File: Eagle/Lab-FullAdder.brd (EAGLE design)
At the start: 50 x 50 mm, 69 parts, among them CN1 HD2, Q1 2N3904-1, Q10 2N3904-1, Q11 2N3904-1, Q12 2N3904-1, Q13 2N3904-1, Q14 2N3904-1, Q15 2N3904-1, Q16 2N3904-1, Q17 BC557BH, Q18 BC557BH, Q2 2N3904-1, Q3 2N3904-1, Q4 2N3904-1, Q5 2N3904-1, Q6 2N3904-1, Q7 2N3904-1, Q8 BC557BH, Q9 BC557BH

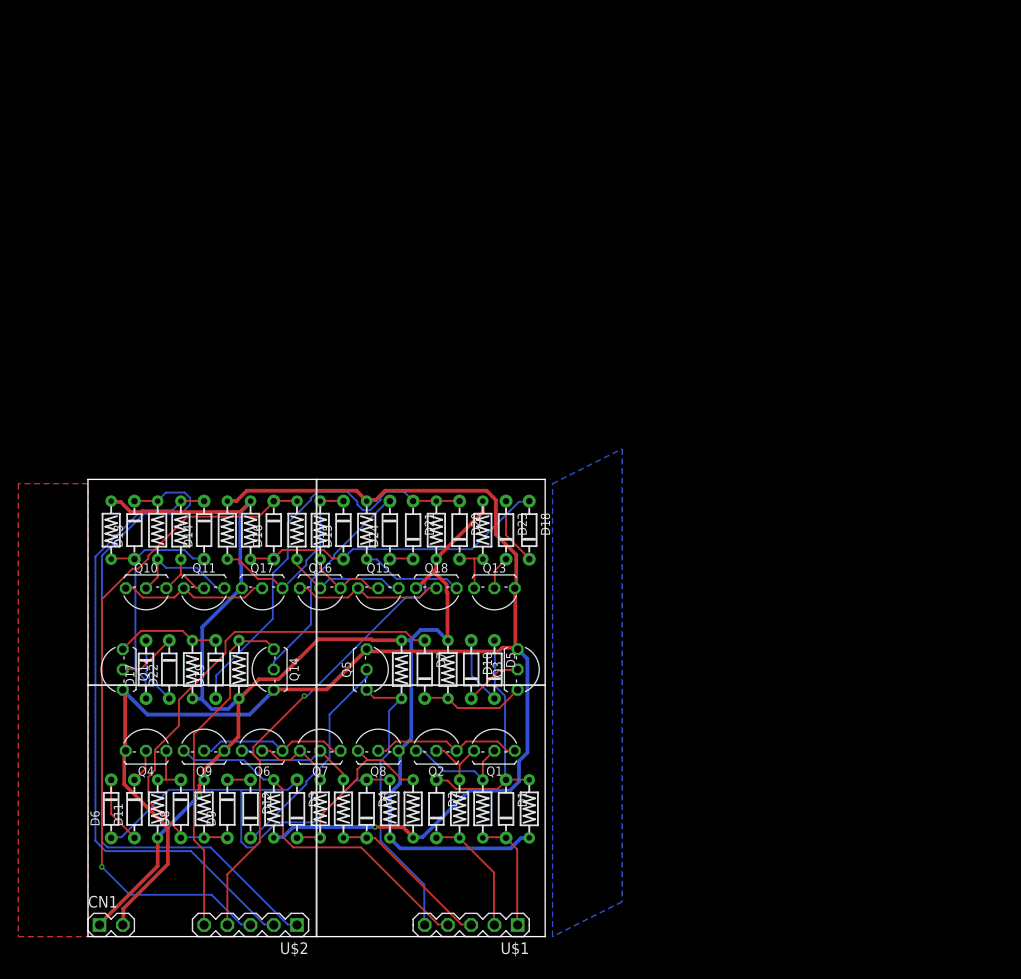
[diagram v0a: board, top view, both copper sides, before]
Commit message: General flush of files
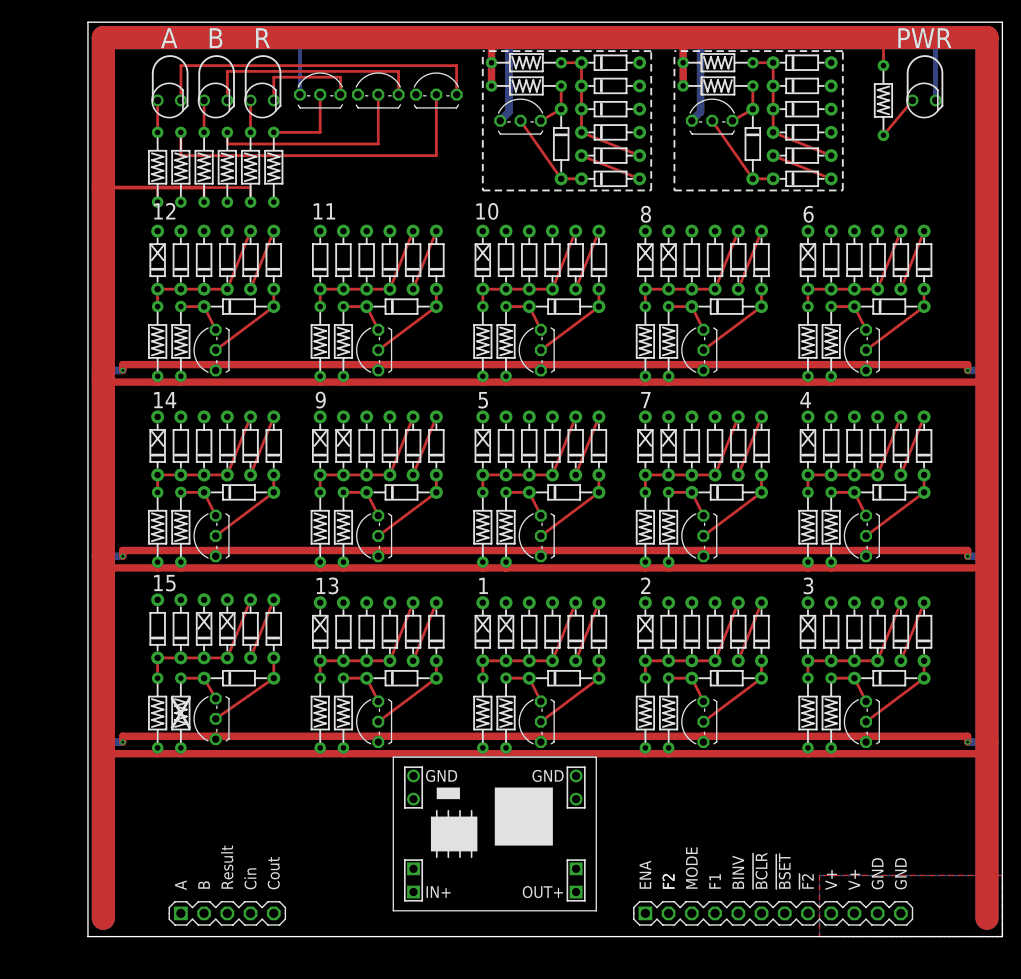
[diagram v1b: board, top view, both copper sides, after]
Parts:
- removed U$2: HD5CN, SmallRoomLabs_ConSwitch:HD5
- added D100, D101, D102, D104, D105, D106, D107, D108, D109, D110, D111, D112, D113, D114, D115, D116, D117, D118, D119, D25, D26, D27, D28, D30, D31, D32, D33, D34, D36, D37, D38, D39, D40, D43, D44, D45, D46, D47, D49, D50, D51, D52, D53, D55, D56, D57, D58, D59, D62, D63, D64, D65, D66, D68, D69, D70, D71, D72, D74, D75, D76, D77, D78, D80, D81, D82, D83, D84, D85, D86, D87, D88, D89, D90, D92, D93, D94, D95, D96, D98, D99: DIODE-6.3, SmallRoomLabs_Semiconductor:DO35-6.3
- added D103, D29, D35, D41, D42, D48, D54, D60, D61, D67, D73, D79, D91, D97: DIODE-7.6, SmallRoomLabs_Semiconductor:DO35-7.6
- added LD1, LD2, LD3, LD4: LED-RA, SmallRoomLabs_Led:3MMRA
- added Q19, Q20: 2N3904-1, SmallRoomLabs_Semiconductor:TO92BH
- added R25, R26, R27, R28, R29, R30, R31, R32, R33, R34, R35, R38, R39, R40, R41, R42, R43: R1/8-7.6MM, SmallRoomLabs_Discrete:R0125-7.6
- added VR1: SMPS, SmallRoomLabs_Battery:BUCK1722
- CN1: value HD2 -> HD12; device SmallRoomLabs_ConSwitch:HD2 -> SmallRoomLabs_ConSwitch:HD12
- D11, D17, D23: value DIODE-6.3 -> DIODE-7.6; device SmallRoomLabs_Semiconductor:DO35-6.3 -> SmallRoomLabs_Semiconductor:DO35-7.6
- Q17, Q18, Q8, Q9: value BC557BH -> 2N3904-1
- R1, R10, R11, R12, R13, R14, R15, R16, R17, R18, R19, R2, R20, R21, R22, R23, R24, R3, R4, R5, R6, R7, R8, R9: value R1/8-6MM -> R1/8-7.6MM; device SmallRoomLabs_Discrete:R0125-6.3 -> SmallRoomLabs_Discrete:R0125-7.6
- moved D22 86.1 mm to (91.4, 53.7), turned to 270 degrees
- moved Q4 82.2 mm to (85.1, 43.8), turned to 90 degrees
- moved D17 81.3 mm to (87.6, 28.3), turned to 180 degrees
- moved D13 79.5 mm to (83.8, 33.3), turned to 270 degrees
- moved Q6 79.3 mm to (85.1, 64.1), turned to 90 degrees
- moved R10 77.5 mm to (78.7, 44.8)
- moved R11 75.2 mm to (81.3, 44.8), turned to 270 degrees
- moved D14 74.5 mm to (86.4, 33.3), turned to 270 degrees
- moved D19 74.0 mm to (83.8, 53.7), turned to 270 degrees
- moved CN1 72.4 mm to (74.9, 2.54)
- moved D16 72.0 mm to (91.4, 33.3), turned to 270 degrees
- moved R17 69.2 mm to (81.3, 65.1), turned to 270 degrees
- moved D12 66.4 mm to (81.3, 33.3)
- moved D11 66.3 mm to (69.8, 28.3), turned to 180 degrees
- moved R16 64.4 mm to (78.7, 65.1)
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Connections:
- removed net A2: D13.C, R14.2, U$2.P$1
- removed net B2: D14.C, R15.2, U$2.P$2
- removed net CI: D4.C, R7.1, U$1.P$3
- removed net CI2: D16.C, R19.1, U$2.P$3
- removed net CO: Q5.3, R12.1, U$1.P$5
- removed net CO2: Q14.3, R24.1, U$2.P$5
- removed net N$19: D11.C, Q4.2
- removed net S: Q9.1, R8.2, U$1.P$4
- removed net S2: Q18.1, R20.2, U$2.P$4
- new net !BCLR: CN1.P$6, D14.A, D7.A
- new net !BSET: CN1.P$7, D20.A
- new net !F2: CN1.P$8, D32.A
- new net BINV: CN1.P$5, D12.A, D2.A
- new net CIN: D36.A, D55.A, U$1.P$4
- new net COUT: D73.C, Q13.3, R18.1, U$1.P$5
- new net ENA: CN1.P$1, D68.A, D98.A
- new net F1: CN1.P$4, D25.A
- new net F2: CN1.P$2, D113.A, D63.A
- new net G10OUT: D114.A, D60.C, D62.A, D69.A, Q10.3, R29.1
- new net G11OUT: D61.C, D74.A, Q11.3, R6.1
- new net G12OUT: D67.C, D75.A, Q12.3, R12.1
- new net G14OUT: D119.A, D79.C, Q14.3, R24.1
- new net G1OUT: D13.A, D41.C, D8.A, Q1.3, R3.1
- new net G2OUT: D11.C, D18.A, Q2.3, R5.1
- new net G3OUT: D17.C, D19.A, Q3.3, R8.1
- new net G4OUT: D23.C, D26.A, D31.A, D45.A, Q4.3, R11.1
- new net G5OUT: D29.C, D38.A, D44.A, D70.A, Q5.3, R14.1
- new net G6OUT: D35.C, D76.A, Q6.3, R17.1
- new net G7OUT: D42.C, D50.A, Q7.3, R20.1
- new net G8OUT: D48.C, D51.A, Q8.3, R23.1
- new net G9OUT: D54.C, D57.A, D64.A, Q9.3, R26.1
- new net MODE: CN1.P$3, D3.A, D56.A
- new net N$37: D27.C, D28.A
- new net N$38: D28.C, D29.A, Q5.2
- new net N$39: D87.A
- new net N$40: D88.A
- new net N$41: D81.A
- new net N$42: D117.C, D86.C, D87.C, D88.C, D89.A, R38.1
- new net N$43: D89.C, D90.A
- new net N$44: D109.C, D30.C, D31.C, D32.C, D33.A, R16.1
- new net N$45: D33.C, D34.A
- new net N$46: D34.C, D35.A, Q6.2
- new net N$47: D90.C, D91.A, Q19.2
- new net N$48: D118.C, D92.C, D93.C, D94.C, D95.A, R40.1
- new net N$49: D95.C, D96.A
- new net N$50: D96.C, D97.A, Q20.2
- new net N$51: D100.C, D101.A, D119.C, D98.C, D99.C, R42.1
- new net N$52: D112.C, D37.C, D38.C, D39.A, D83.C, R19.1
- new net N$53: D39.C, D40.A
- new net N$54: D40.C, D42.A, Q7.2
- new net N$55: D101.C, D102.A
- new net N$56: D102.C, D103.A, Q15.2
- new net N$57: D115.C, D62.C, D63.C, D64.C, D65.A, R9.1
- new net N$58: D82.A
- new net N$59: D83.A
- new net N$60: D110.C, D44.C, D45.C, D46.A, D81.C, R22.1
- new net N$61: D46.C, D47.A
- new net N$62: D47.C, D48.A, Q8.2
- new net N$63: D85.A
- new net N$64: D65.C, D66.A
- new net N$65: D66.C, D67.A, Q12.2
- new net N$66: D84.A
- new net N$67: D104.A
- new net N$68: D111.C, D50.C, D51.C, D52.A, D82.C, R25.1
- new net N$69: D52.C, D53.A
- new net N$70: D53.C, D54.A, Q9.2
- new net N$71: D105.A
- new net N$72: D106.A
- new net N$73: D108.A
- new net N$74: D107.A
- new net N$75: D109.A
- new net N$76: D104.C, D55.C, D56.C, D57.C, D58.A, R28.1
- new net N$77: D58.C, D59.A
- new net N$78: D59.C, D60.A, Q10.2
- new net N$79: D110.A
- new net N$80: D111.A
- new net N$81: D112.A
- new net N$82: D116.C, D68.C, D69.C, D70.C, D71.A, R15.1
- new net N$83: D71.C, D72.A
- new net N$84: D72.C, D73.A, Q13.2
- new net N$85: D116.A
- new net N$86: D115.A
- new net N$88: D118.A
- new net N$89: D74.C, D75.C, D76.C, D77.A, D80.C, R21.1
- new net N$90: D77.C, D78.A
- new net N$91: D78.C, D79.A, Q14.2
- new net N$92: D117.A
- new net RES: D103.C, Q15.3, R33.2, R43.1, U$1.P$3
- new net VIN: VR1.IN@1, VR1.IN@2
- new net VOUT: VR1.OUT@1, VR1.OUT@2
- net A: now also D24.A, D30.A, D37.A, R35.2; no longer D1.C, R2.2
- net B: now also D1.A, D6.A, R34.2; no longer D2.C, R3.2
- net GND: now also CN1.P$11, CN1.P$12, LD4.C, Q1.1, Q10.1, Q11.1, Q15.1, Q16.1, Q17.1, Q18.1, Q19.1, Q2.1, Q20.1, Q6.1, Q7.1, Q8.1, Q9.1, VR1.GND@1, VR1.GND@2, VR1.GND@3, VR1.GND@4; no longer CN1.P$2, R17.2, R20.1, R5.2, R8.1
- net N$1: now also LD1.A, R27.1; no longer D1.A, D2.A, D5.A, R1.1
- net N$10: now also LD2.C, Q16.3; no longer Q6.2, Q7.1, R6.2
- net N$11: now also LD1.C, Q17.3; no longer D3.C, Q8.1, R5.1, R6.1
- net N$12: now also D108.C, D6.C, D7.C, D8.C, D9.A, R2.1; no longer D3.A, D4.A, D6.A, R4.2
- net N$13: now also D10.A, D9.C; no longer D10.C, Q3.2
- net N$14: now also D10.C, D11.A, Q2.2; no longer Q10.2, Q11.1, R14.1
- net N$15: now also Q18.2, R33.1; no longer Q6.3, Q7.3, Q9.2
- net N$16: now also D113.C, D114.C, D3.C, D36.C, D43.A, R4.1; no longer Q10.1, Q11.2, R15.1
- net N$17: now also Q16.2, R34.1; no longer D7.A, D8.A, D9.A, R11.1
- net N$18: now also Q17.2, R35.1; no longer D12.C, Q5.2
- net N$2: now also LD2.A, R30.1; no longer Q1.2, Q2.1, R2.1
- net N$20: now also D105.C, D12.C, D13.C, D14.C, D15.A, R7.1; no longer D7.C, Q3.3, R9.1
- net N$21: now also D15.C, D16.A; no longer D8.C, Q4.3, R10.1
- net N$22: now also D16.C, D17.A, Q3.2; no longer Q10.3, Q11.3, Q17.2
- net N$23: now also D99.A; no longer Q15.1, Q16.2, R19.2
- net N$24: now also D43.C, D49.A; no longer Q15.2, Q16.1, R18.2
- net N$25: now also D100.A; no longer D15.C, Q17.1, R17.1, R18.1
- net N$26: now also D92.A; no longer D15.A, D16.A, D18.A, R16.2
- net N$27: now also D93.A; no longer Q15.3, Q16.3, Q18.2
- net N$28: now also D107.C, D18.C, D19.C, D20.C, D21.A, R10.1; no longer D22.C, Q12.2
- net N$29: now also D21.C, D22.A; no longer D23.C, Q13.2
- net N$3: now also LD3.A, R31.1; no longer Q1.1, Q2.2, R3.1
- net N$30: now also D22.C, D23.A, Q4.2; no longer D19.C, Q12.3, R21.1
- net N$31: now also D94.A; no longer D20.C, Q13.3, R22.1
- net N$32: now also D49.C, D61.A, Q11.2; no longer D19.A, D20.A, D21.A, R23.1
- net N$33: now also D97.C, Q20.3, R41.1; no longer D24.C, Q14.2
- net N$34: now also D91.C, Q19.3, R39.1; no longer D17.C, D22.A
- net N$35: now also D86.A; no longer D18.C, D23.A
- net N$36: now also D106.C, D24.C, D25.C, D26.C, D27.A, R13.1; no longer D21.C, D24.A
- net N$4: now also D1.C, D2.C, D4.A, D84.C, D85.C, R1.1; no longer D10.A, D5.C
- net N$5: now also D4.C, D5.A; no longer D11.A, D6.C
- net N$6: now also D41.A, D5.C, Q1.2; no longer D12.A, D9.C
- net N$7: now also LD4.A, R32.1; no longer D13.A, D14.A, D17.A, R13.1
- net N$8: now also D80.A; no longer Q1.3, Q2.3, Q8.2
- net N$9: now also LD3.C, Q18.3; no longer Q6.1, Q7.2, R7.2
- net V+: now also CN1.P$10, CN1.P$9, R14.2, R15.2, R16.2, R17.2, R18.2, R19.2, R2.2, R20.2, R25.2, R26.2, R27.2, R28.2, R29.2, R3.2, R30.2, R31.2, R32.2, R38.2, R39.2, R4.2, R40.2, R41.2, R42.2, R43.2, R5.2, R6.2, R7.2, R8.2; no longer CN1.P$1, Q17.3, Q18.3, Q8.3, Q9.3, R16.1, R4.1
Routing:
- net V+: track 163.9 -> 659.2 mm, vias 1 -> 0
- net GND: track 172.3 -> 631.4 mm, vias 1 -> 6
- net A2: track 75.9 -> 0.00 mm
- net CI2: track 74.2 -> 0.00 mm, vias 1 -> 0
- net B2: track 68.9 -> 0.00 mm
- net S2: track 59.6 -> 0.00 mm, vias 1 -> 0
- net S: track 39.9 -> 0.00 mm
- net CO2: track 37.9 -> 0.00 mm
- net N$32: track 45.3 -> 9.84 mm
- net N$26: track 34.2 -> 0.00 mm
- net N$12: track 48.6 -> 16.4 mm
- net CO: track 32.0 -> 0.00 mm
- net N$17: track 54.5 -> 23.2 mm
- net N$1: track 26.9 -> 3.49 mm
- net N$7: track 27.0 -> 4.96 mm
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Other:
- board size 50 x 50 mm -> 100 x 100 mm
- board text added: "!BCLR"
- board text added: "!BSET"
- board text added: "!F2"
- board text added: "1"
- board text added: "10"
- board text added: "11"
- board text added: "12"
- board text added: "13"
- board text added: "14"
- board text added: "15"
- board text added: "2"
- board text added: "3"
- board text added: "4"
- board text added: "5"
- board text added: "6"
- board text added: "7"
- board text added: "8"
- board text added: "9"
- board text added: "A"
- board text added: "B"
- board text added: "BINV"
- board text added: "Cin"
- board text added: "Cout"
- board text added: "ENA"
- board text added: "F1"
- board text added: "F2"
- board text added: "GND"
- board text added: "MODE"
- board text added: "PWR"
- board text added: "R"
- board text added: "Result"
- board text added: "V+"
